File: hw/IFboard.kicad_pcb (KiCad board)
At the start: 2 copper layers, 110 x 65.1 mm, 99 parts, among them J1 USB_C_Receptacle_USB2.0_16P, J10 IcoTec_36650.2, J2 Phoenix_1881561, J3 Conn_ARM_SWD_TagConnect_TC203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, J4 Phoenix_1881561, J5 Phoenix_1881561, J6 Phoenix_1881561, J7 IcoTec_36650.2, J8 IcoTec_36650.2, J9 IcoTec_36650.2, SW3 SW_Push, SW4 SW_Push, SW5 SW_Push, SW6 SW_Push, U2 XC6206P332MR-G, U3 TCAN3413DR, U4 ST4E1240DT, U5 MAX232ESE+T, U6 STM32G0B1CBTx, U7 ER_OLEDM0.91_1x-I2C

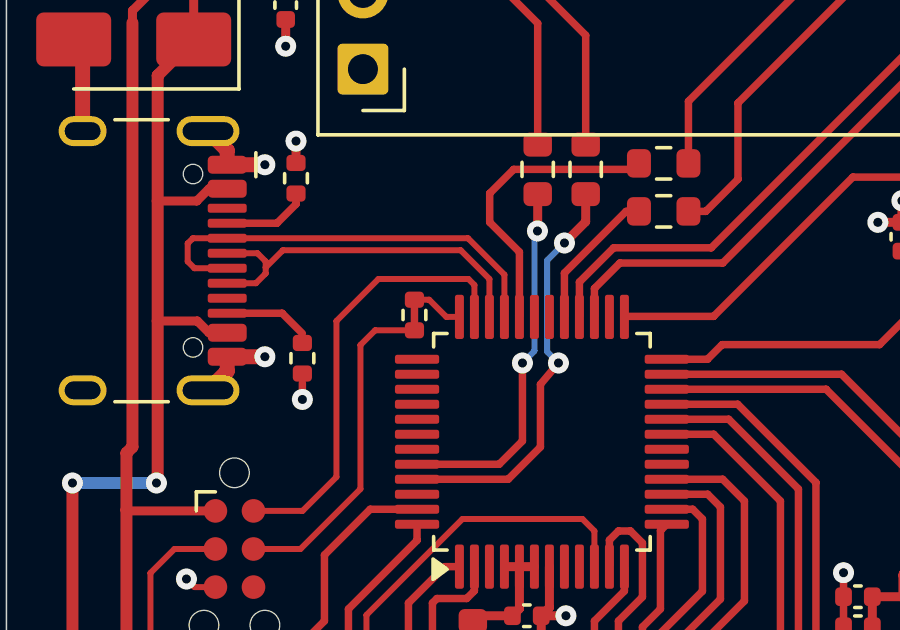
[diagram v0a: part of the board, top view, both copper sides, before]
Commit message: cleanup
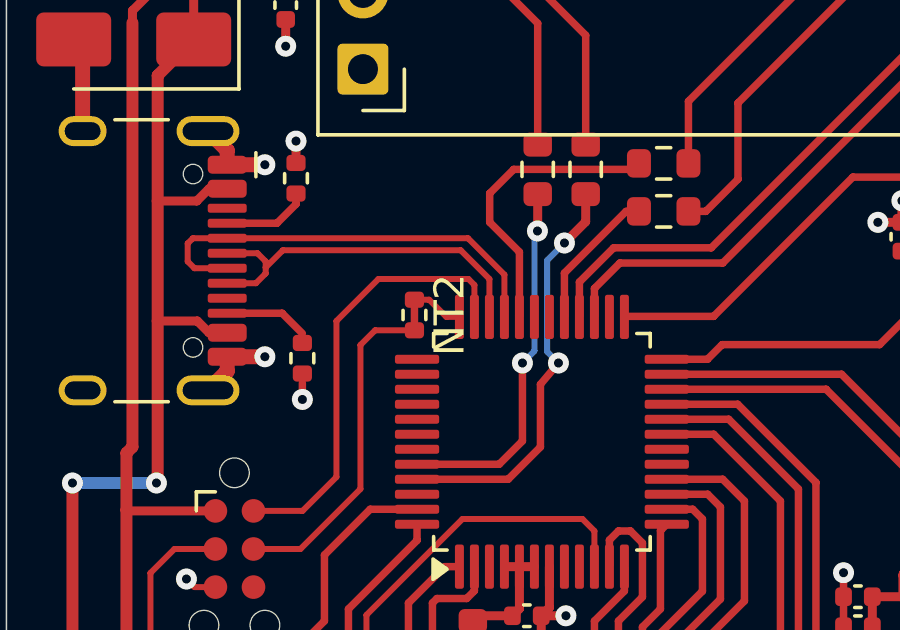
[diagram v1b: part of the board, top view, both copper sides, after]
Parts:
- D13, D14: footprint PZL:TVS_PESD2CANFD24V-UX -> PZ:TVS_PESD2CANFD24V-UX
- L1, L2: footprint PZL:L_Wurth_WE-SL2-74422x -> PZ:L_Wurth_WE-SL2-74422x
- NT2: footprint Franz:R_0402_1005Metric_solderjmp_short -> PZ:R_0402_1005Metric_solderjmp_short
- TP1, TP10, TP11: value TestPoint -> TestPoint_Keystone_5019; footprint PZL:TestPoint_Keystone_5019_Miniature -> PZ:TestPoint_Keystone_5019_Miniature
- U7: footprint PZL:ER_OLEDM0.91_1x-I2C -> PZ:ER_OLEDM0.91_1x-I2C
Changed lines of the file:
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@@
 			)
 		)
-		(attr through_hole)
+		(attr through_hole dnp)
 		(duplicate_pad_numbers_are_jumpers no)
 		(fp_line
@@
 			)
 		)
-		(attr through_hole)
+		(attr through_hole dnp)
 		(duplicate_pad_numbers_are_jumpers no)
 		(fp_line
@@
 		)
 	)
-	(footprint "PZL:TestPoint_Keystone_5019_Miniature"
+	(footprint "PZ:TestPoint_Keystone_5019_Miniature"
 		(layer "F.Cu")
 		(at 91.44 85.330344 90)
@@
 			)
 		)
-		(property "Value" "TestPoint"
+		(property "Value" "TestPoint_Keystone_5019"
 			(at 0 2.25 90)
 			(layer "F.Fab")
@@
 			)
 		)
-		(property "LCSC Part #" ""
+		(property "LCSC Part #" "C238131"
 			(at 0 0 90)
 			(unlocked yes)
@@
 		)
 	)
-	(footprint "PZL:TestPoint_Keystone_5019_Miniature"
+	(footprint "PZ:TestPoint_Keystone_5019_Miniature"
 		(layer "F.Cu")
 		(at 91.44 55.226 -90)
@@
 			)
 		)
-		(property "Value" "TestPoint"
+		(property "Value" "TestPoint_Keystone_5019"
 			(at 0 2.25 270)
 			(layer "F.Fab")
@@
 			)
 		)
-		(property "LCSC Part #" ""
+		(property "LCSC Part #" "C238131"
 			(at 0 0 270)
 			(unlocked yes)
@@
 			)
 		)
-		(attr through_hole)
+		(attr through_hole dnp)
 		(duplicate_pad_numbers_are_jumpers no)
 		(fp_line
@@
 		)
 	)
-	(footprint "PZL:TVS_PESD2CANFD24V-UX"
+	(footprint "PZ:TVS_PESD2CANFD24V-UX"
 		(layer "F.Cu")
 		(at 109.1946 74.8856 180)
@@
 			)
 		)
-		(attr through_hole)
+		(attr through_hole dnp)
 		(duplicate_pad_numbers_are_jumpers no)
 		(fp_line
@@
 		)
 	)
-	(footprint "PZL:TVS_PESD2CANFD24V-UX"
+	(footprint "PZ:TVS_PESD2CANFD24V-UX"
 		(layer "F.Cu")
 		(at 108.966 90.532 180)
@@
 		)
 	)
-	(footprint "PZL:L_Wurth_WE-SL2-74422x"
+	(footprint "PZ:L_Wurth_WE-SL2-74422x"
 		(layer "F.Cu")
 		(at 94.0054 75.0888)
@@
 			)
 		)
-		(property "LCSC Part #" ""
+		(property "LCSC Part #" "C2651122"
 			(at 0 0 0)
 			(unlocked yes)
@@
 		)
 	)
-	(footprint "PZL:ER_OLEDM0.91_1x-I2C"
+	(footprint "PZ:ER_OLEDM0.91_1x-I2C"
 		(locked yes)
 		(layer "F.Cu")
@@
 			)
 		)
-		(attr smd exclude_from_bom)
+		(attr smd)
 		(duplicate_pad_numbers_are_jumpers no)
 		(fp_line
@@
 		)
 	)
-	(footprint "Franz:R_0402_1005Metric_solderjmp_short"
+	(footprint "PZ:R_0402_1005Metric_solderjmp_short"
 		(layer "F.Cu")
 		(at 64.527 77.024 -90)
@@
 		(tags "resistor")
 		(property "Reference" "NT2"
-			(at 0 -1.17 90)
+			(at 0 -1.17 270)
 			(layer "F.SilkS")
-			(hide yes)
 			(effects
 				(font
@@
 		)
 		(property "Value" "NetTie_2"
-			(at 0 1.17 90)
+			(at 0 1.17 270)
 			(layer "F.Fab")
-			(hide yes)
 			(effects
 				(font
@@
 			)
 		)
-		(attr smd exclude_from_bom dnp)
+		(attr smd exclude_from_bom)
 		(duplicate_pad_numbers_are_jumpers no)
 		(fp_line
@@
 		)
 		(fp_text user "${REFERENCE}"
-			(at 0 0 90)
+			(at 0 0 270)
 			(layer "F.Fab")
 			(effects
@@
 		)
 	)
-	(footprint "PZL:L_Wurth_WE-SL2-74422x"
+	(footprint "PZ:L_Wurth_WE-SL2-74422x"
 		(layer "F.Cu")
 		(at 87.503 90.7352)
@@
 			)
 		)
-		(property "LCSC Part #" ""
+		(property "LCSC Part #" "C2651122"
 			(at 0 0 0)
 			(unlocked yes)
@@
 		)
 	)
-	(footprint "PZL:TestPoint_Keystone_5019_Miniature"
+	(footprint "PZ:TestPoint_Keystone_5019_Miniature"
 		(layer "F.Cu")
 		(at 91.44 109.424 90)
@@
 			)
 		)
-		(property "Value" "TestPoint"
+		(property "Value" "TestPoint_Keystone_5019"
 			(at 0 2.25 90)
 			(layer "F.Fab")
@@
 			)
 		)
-		(property "LCSC Part #" ""
+		(property "LCSC Part #" "C238131"
 			(at 0 0 90)
 			(unlocked yes)
